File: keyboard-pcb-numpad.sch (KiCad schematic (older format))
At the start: 15 parts

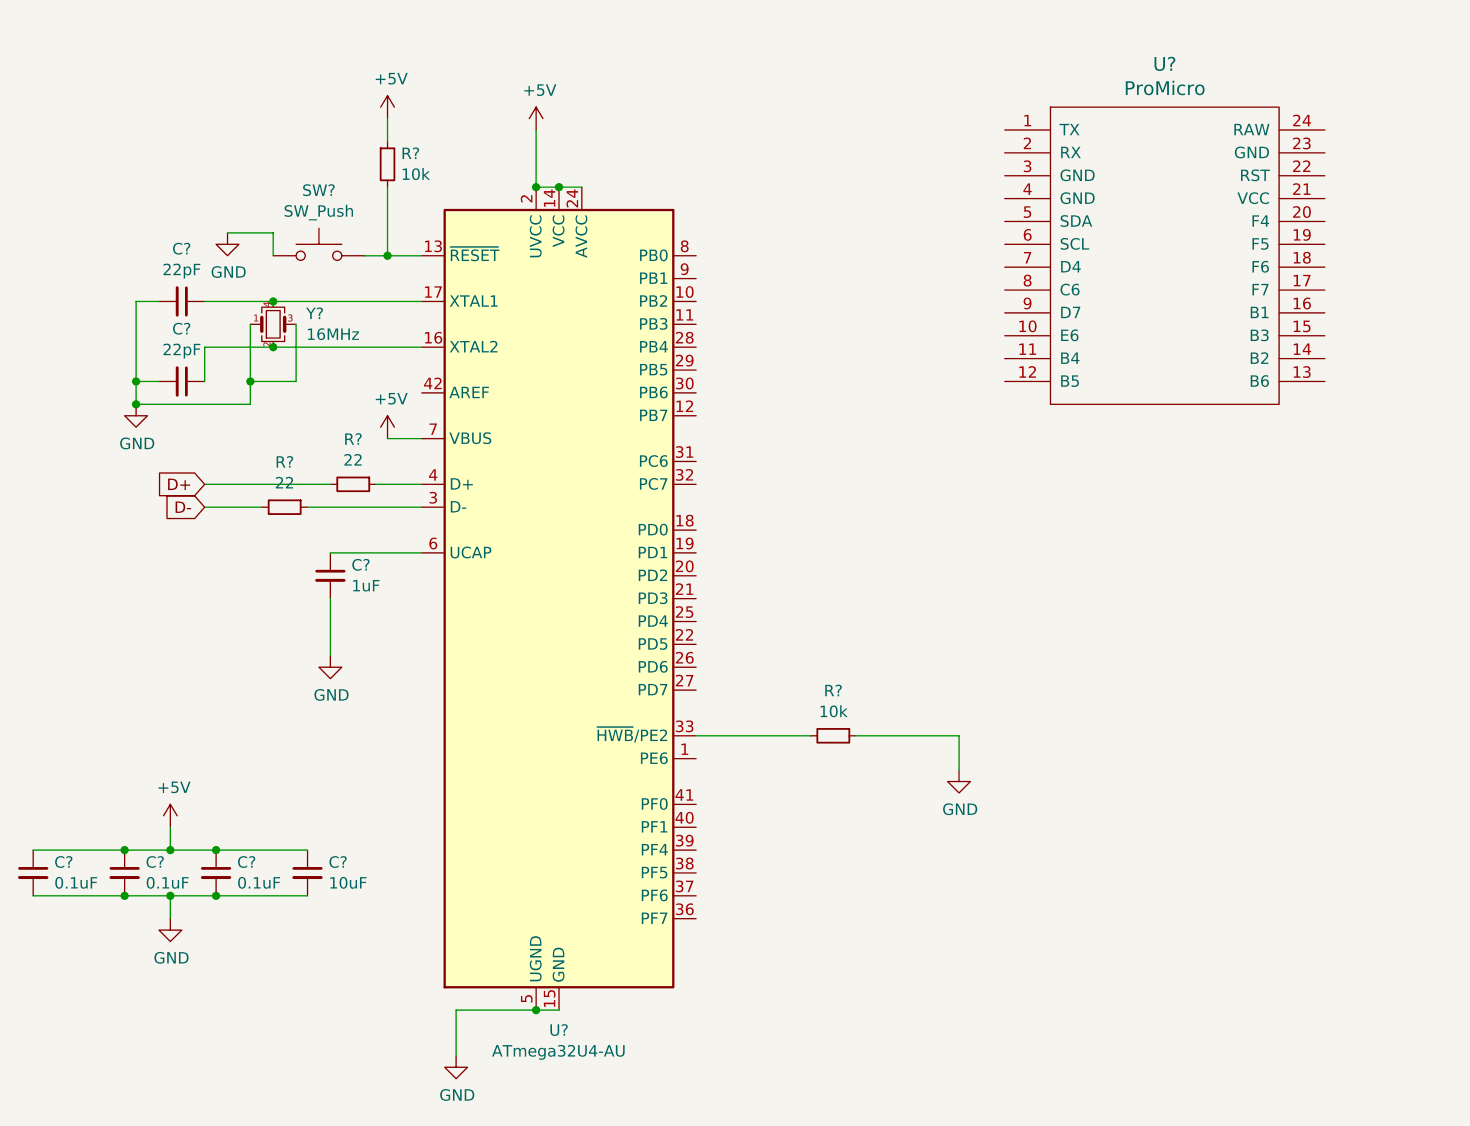
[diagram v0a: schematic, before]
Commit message: feat: complete electrical setup
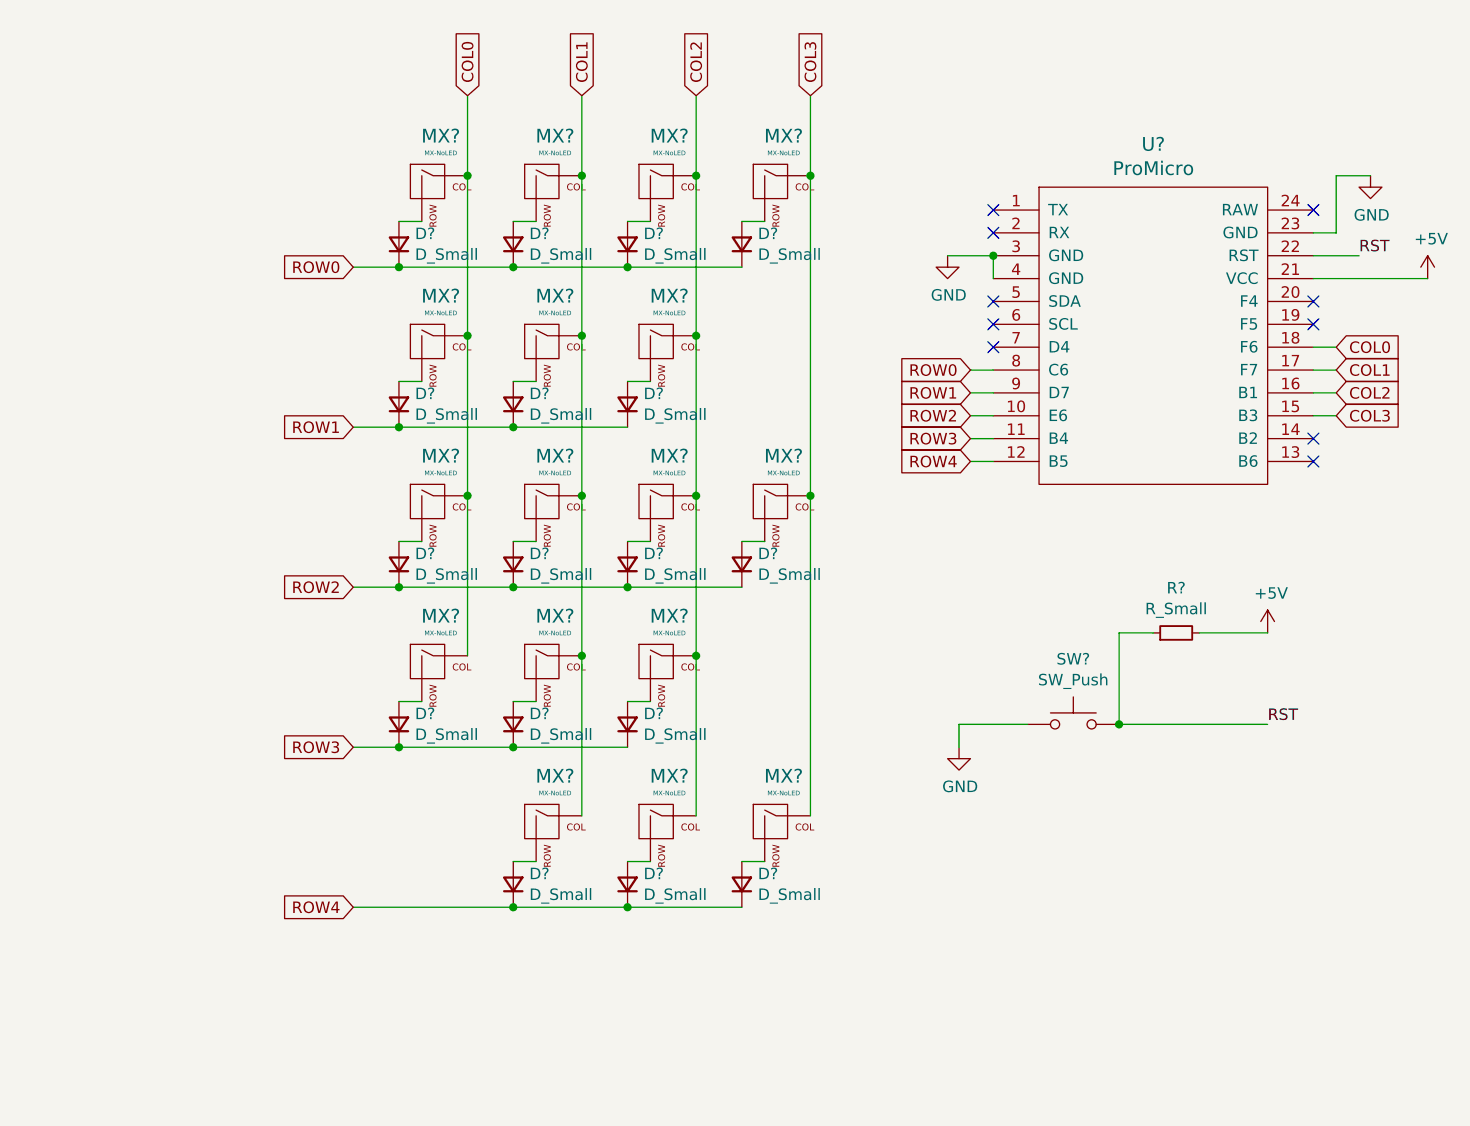
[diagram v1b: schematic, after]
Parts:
- removed C?: 1uF, symbol Device:C_Small
- removed C? (x3): 0.1uF, symbol Device:C_Small
- removed C?: 10uF, symbol Device:C_Small
- removed C? (x2): 22pF, symbol Device:C_Small
- removed R? (x2): 10k, symbol Device:R_Small
- removed R? (x2): 22, symbol Device:R_Small
- removed SW?: SW_Push, symbol Switch:SW_Push
- removed U?: ATmega32U4-AU, Package_QFP:TQFP-44_10x10mm_P0.8mm, symbol MCU_Microchip_ATmega:ATmega32U4-AU
- removed Y?: 16MHz, symbol Device:Crystal_GND24_Small
- added D? (x17): D_Small, symbol Device:D_Small
- added MX? (x17): MX-NoLED, symbol MX_Alps_Hybrid:MX-NoLED
- added R?: R_Small, symbol Device:R_Small
- added SW?: SW_Push, symbol Switch:SW_Push
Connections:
- net +5V: now also U?.21 (VCC), R?.2
- net GND: now also U?.23 (GND), U?.3 (GND), U?.4 (GND), SW?.1
- net ROW2: now reaches U?.10 (E6)
- net ROW2: now also D?.1 (K), D?.1 (K), D?.1 (K), D?.1 (K)
- net ROW3: now reaches U?.11 (B4)
- net ROW3: now also D?.1 (K), D?.1 (K), D?.1 (K)
- net ROW4: now reaches U?.12 (B5)
- net ROW4: now also D?.1 (K), D?.1 (K), D?.1 (K)
- net COL3: now reaches U?.15 (B3)
- net COL3: now also MX?.1 (COL), MX?.1 (COL), MX?.1 (COL)
- net COL2: now reaches U?.16 (B1)
- net COL2: now also MX?.1 (COL), MX?.1 (COL), MX?.1 (COL), MX?.1 (COL), MX?.1 (COL)
- net COL1: now reaches U?.17 (F7)
- net COL1: now also MX?.1 (COL), MX?.1 (COL), MX?.1 (COL), MX?.1 (COL), MX?.1 (COL)
- net COL0: now reaches U?.18 (F6)
- net COL0: now also MX?.1 (COL), MX?.1 (COL), MX?.1 (COL), MX?.1 (COL)
- net RST: now reaches U?.22 (RST)
- net RST: now also R?.1, SW?.2
- net ROW0: now reaches U?.8 (C6)
- net ROW0: now also D?.1 (K), D?.1 (K), D?.1 (K), D?.1 (K)
- net ROW1: now reaches U?.9 (D7)
- net ROW1: now also D?.1 (K), D?.1 (K), D?.1 (K)
- new net: D?.2 (A), MX?.2 (ROW) (x17)
- no-connect marks 0 -> 10
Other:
- moved on the sheet: U?
